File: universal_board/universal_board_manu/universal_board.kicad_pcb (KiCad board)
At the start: 2 copper layers, 83.3 x 92.5 mm, 54 parts

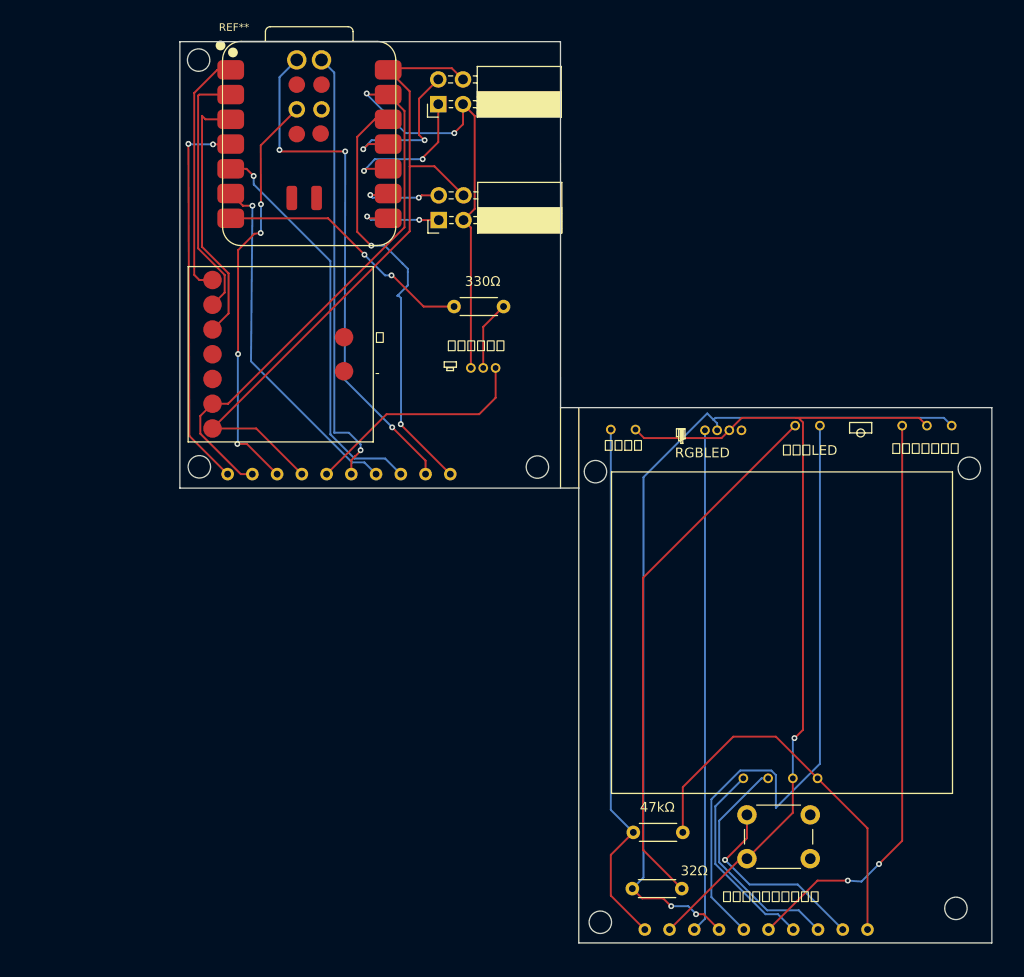
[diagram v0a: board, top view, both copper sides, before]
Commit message: board
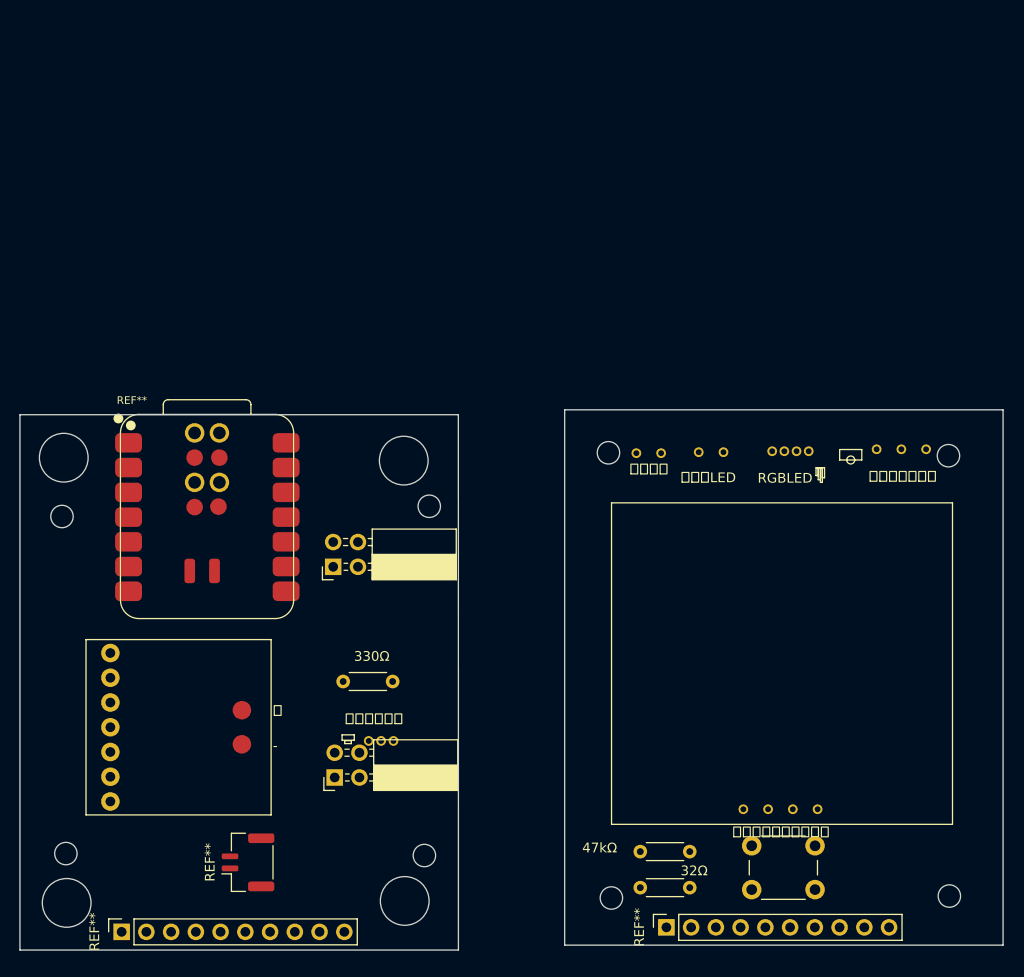
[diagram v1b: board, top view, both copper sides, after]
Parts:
- removed 19 (x2), 20 (x2), 21 (x2), 22 (x2), 23 (x2), 24 (x2), 25 (x2), 26 (x2), 27 (x2): , 
- removed the ? at (150.0, 77.2)
- removed the ? at (192.8, 124.0)
- added REF**: PinSocket_1x10_P2.54mm_Vertical, Connector_PinSocket_2.54mm:PinSocket_1x10_P2.54mm_Vertical, F.Cu at (139.1, 124.2)
- added REF**: PinSocket_1x10_P2.54mm_Vertical, Connector_PinSocket_2.54mm:PinSocket_1x10_P2.54mm_Vertical, F.Cu at (195.0, 123.8)
- added REF**: JST_GH_SM02B-GHS-TB_1x02-1MP_P1.25mm_Horizontal, Connector_JST:JST_GH_SM02B-GHS-TB_1x02-1MP_P1.25mm_Horizontal, F.Cu at (152.1, 117.1)
- moved dawdad 58.2 mm to (161.0, 108.4)
- moved dadada 48.7 mm to (160.8, 86.8)
- moved REF** 40.1 mm to (161.9, 98.5)
- moved 3 39.7 mm to (152.3, 101.9)
- moved 1 39.7 mm to (152.3, 106.9)
- moved 2 39.7 mm to (152.3, 104.4)
- moved 4 39.7 mm to (152.3, 99.3)
- moved 6 39.7 mm to (152.3, 94.2)
- moved 8 39.7 mm to (165.8, 104.6)
- moved ? 39.7 mm to (152.3, 109.5)
- moved 2 39.7 mm to (164.6, 104.2)
- moved 5 39.7 mm to (152.3, 96.8)
- moved 9 39.7 mm to (167.0, 104.6)
- moved ? 39.7 mm to (164.5, 104.6)
- moved 7 39.7 mm to (164.6, 100.7)
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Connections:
- 18 pad : 5V -> 3.3V
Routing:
- net GND: track 187.7 -> 0.00 mm, vias 3 -> 0
- net 5V: track 161.9 -> 0.00 mm, vias 2 -> 0
- net 14: track 105.9 -> 0.00 mm, vias 3 -> 0
- net 4: track 94.7 -> 0.00 mm, vias 2 -> 0
- net 15: track 94.6 -> 0.00 mm, vias 4 -> 0
- net IR: track 90.9 -> 0.00 mm
- net 3.3V: track 84.5 -> 0.00 mm, vias 2 -> 0
- net 13: track 74.2 -> 0.00 mm, vias 4 -> 0
- net 5: track 65.5 -> 0.00 mm, vias 1 -> 0
- net 6: track 57.3 -> 0.00 mm, vias 1 -> 0
- net R_LED: track 55.6 -> 0.00 mm
- net 7: track 26.9 -> 0.00 mm, vias 2 -> 0
- net 3: track 26.8 -> 0.00 mm
- net 2: track 26.5 -> 0.00 mm
- net 1: track 25.5 -> 0.00 mm
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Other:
- board size 83.3 x 92.5 mm -> 100.9 x 55.5 mm
